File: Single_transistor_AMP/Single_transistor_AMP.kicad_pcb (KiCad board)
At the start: 2 copper layers, 24.9 x 27.3 mm, 14 parts, among them J1 AudioJack2_Ground, J2 32V, J3 Signal out, Q1 BC546, Q3 TIP140

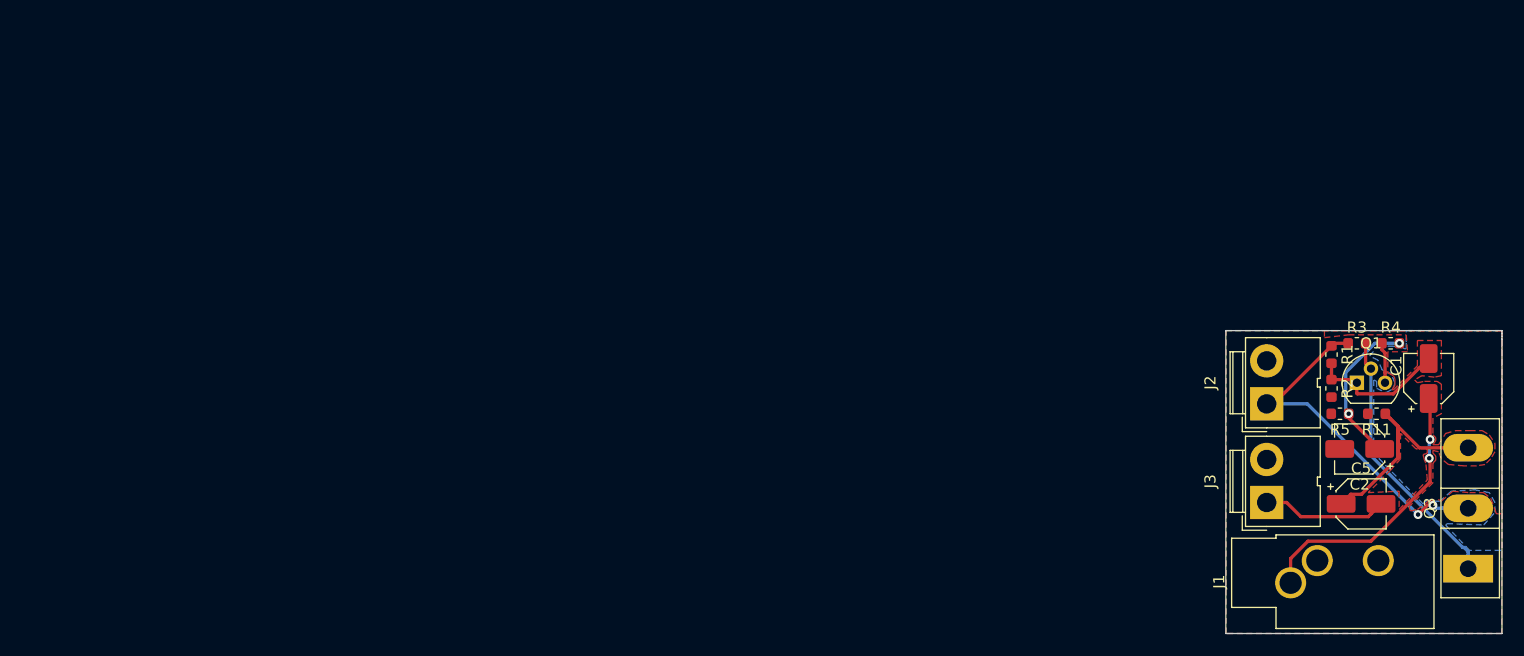
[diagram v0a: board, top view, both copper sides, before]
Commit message: Izpildīts 8 lekcijas MD
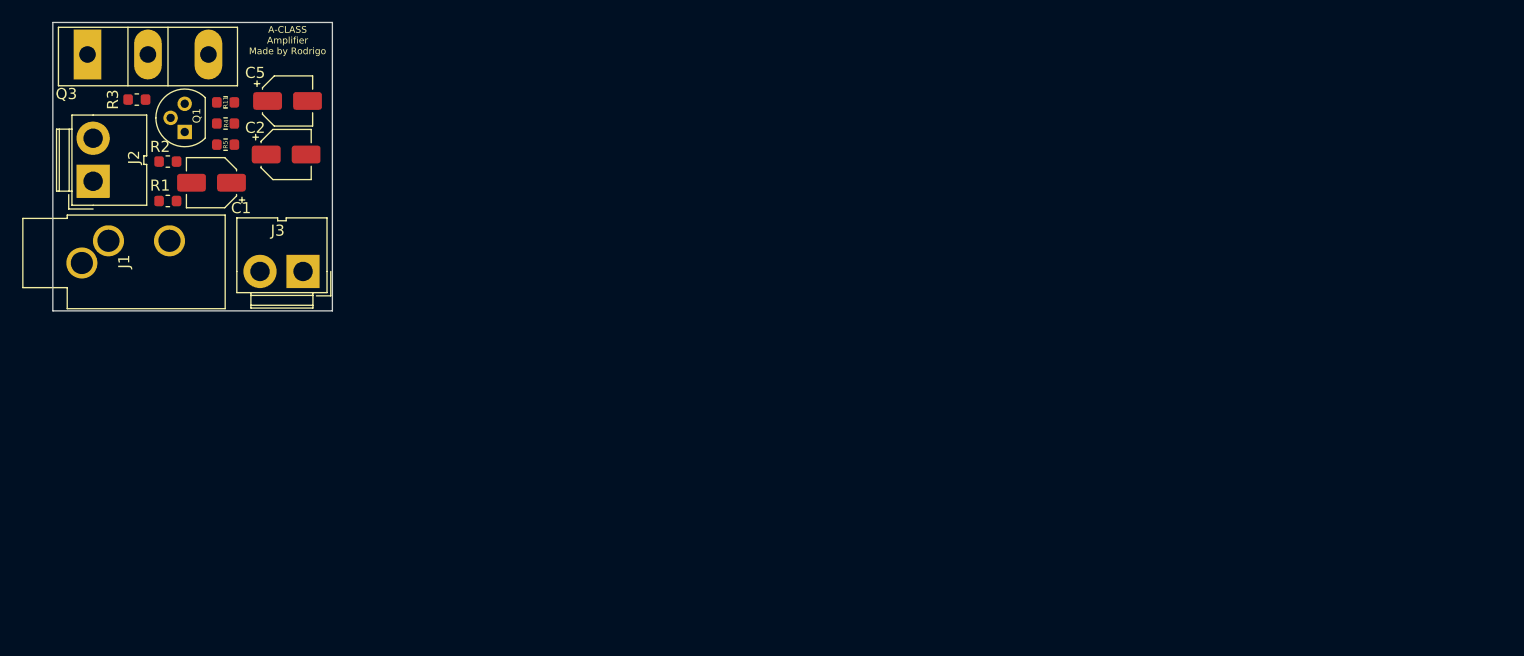
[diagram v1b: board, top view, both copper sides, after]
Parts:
- moved Q3 132.8 mm to (103.1, 111.9), turned to 0 degrees
- moved J1 112.7 mm to (102.6, 130.7)
- moved R3 112.2 mm to (107.6, 116.0)
- moved C1 111.1 mm to (114.3, 123.4), turned to 180 degrees
- moved Q1 108.1 mm to (111.9, 118.9), turned to 90 degrees
- moved J2 107.7 mm to (103.6, 123.3)
- moved R11 107.5 mm to (115.6, 116.2), turned to 0 degrees
- moved R4 106.9 mm to (115.6, 118.1)
- moved R2 106.9 mm to (110.4, 121.5), turned to 180 degrees
- moved R1 105.8 mm to (110.4, 125.1), turned to 0 degrees
- moved C5 103.4 mm to (121.2, 116.1)
- moved R5 103.3 mm to (115.6, 120.0)
- moved C2 100.3 mm to (121.0, 120.9), turned to 0 degrees
- moved J3 89.3 mm to (122.6, 131.4), turned to 180 degrees
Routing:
- net Net-(J2-Pad1): track 34.6 -> 0.00 mm, vias 2 -> 0
- net Net-(Q1-Pad2): track 25.5 -> 0.00 mm
- net Net-(C1-Pad1): track 25.4 -> 0.00 mm, vias 2 -> 0
- net Net-(C5-Pad1): track 22.7 -> 0.00 mm
- net Net-(C2-Pad1): track 14.1 -> 0.00 mm, vias 2 -> 0
- net Net-(C1-Pad2): track 12.6 -> 0.00 mm
- net Net-(C5-Pad2): track 11.3 -> 0.00 mm
- net Net-(Q1-Pad3): track 3.67 -> 0.00 mm
- removed copper zone on B.Cu, net (none)
- removed copper zone on F.Cu, net (none)
- removed copper zone on B.Cu, net GND
- removed copper zone on F.Cu, net GND
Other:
- board size 24.9 x 27.3 mm -> 25.2 x 26 mm
- net class POWER: clearance 0.2 -> 0.5
- board text added: "A-CLASS Amplifier Made by Rodrigo"
